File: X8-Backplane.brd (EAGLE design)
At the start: 101.9 x 101.6 mm, 17 parts

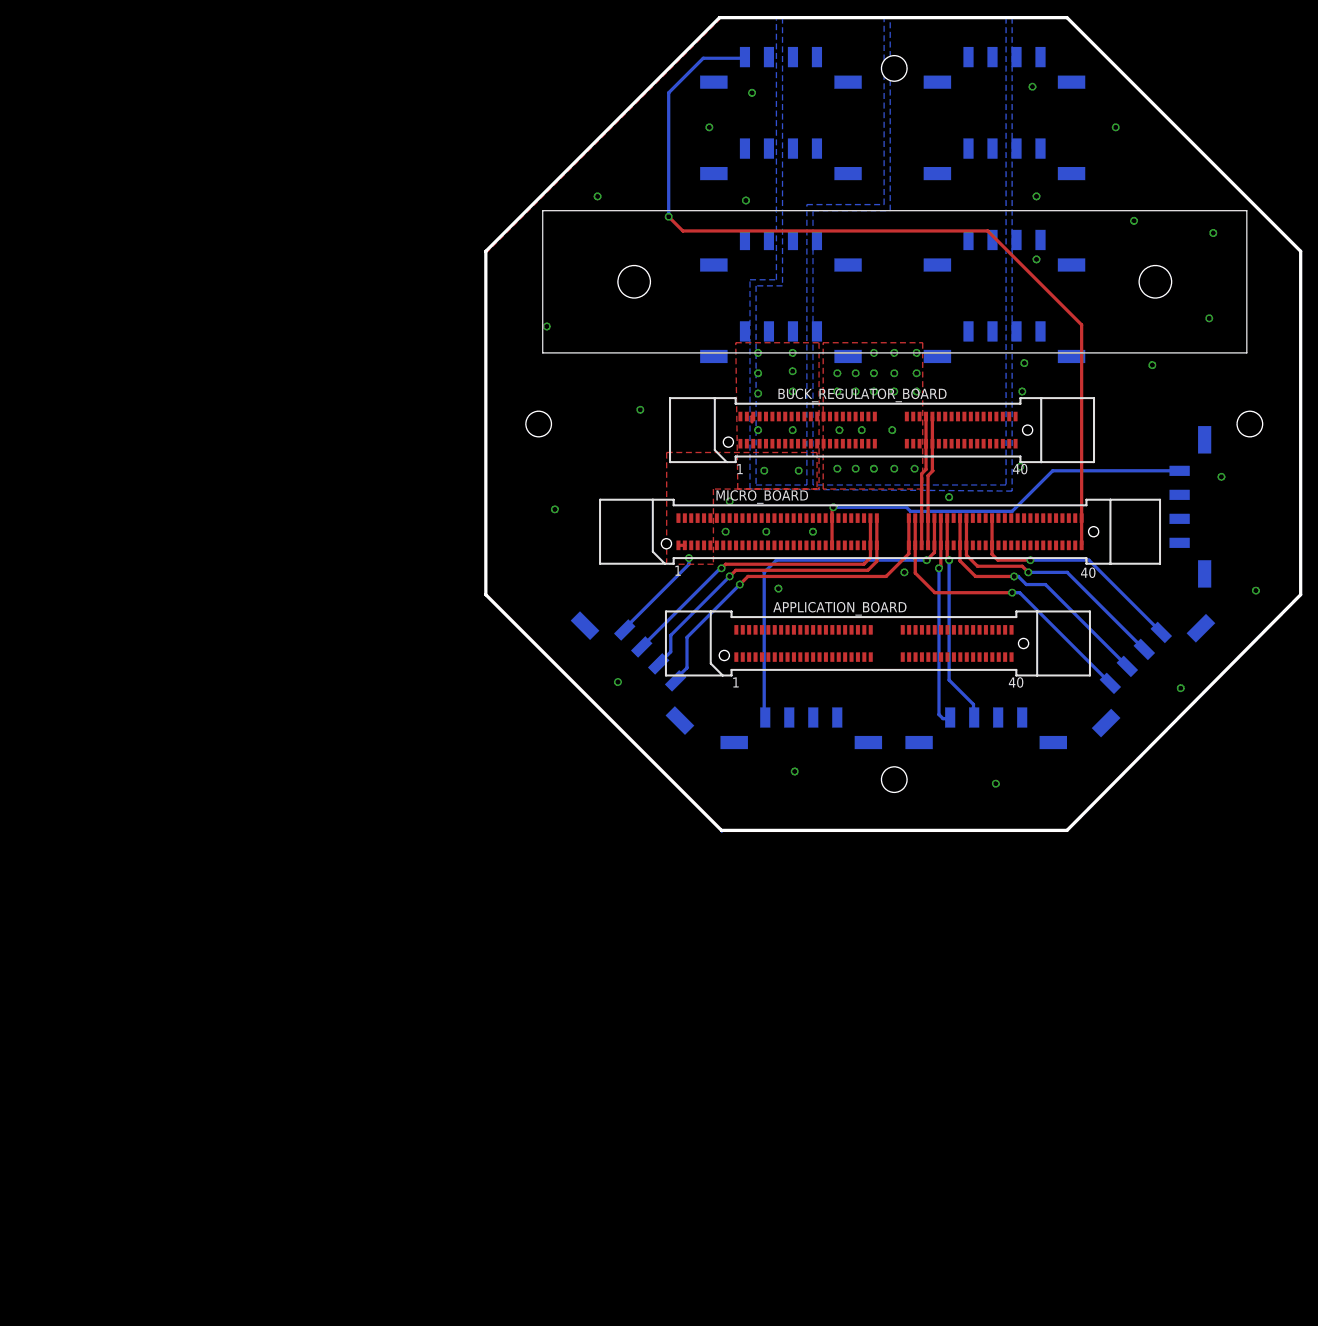
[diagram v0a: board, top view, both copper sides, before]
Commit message: Finished the backplane
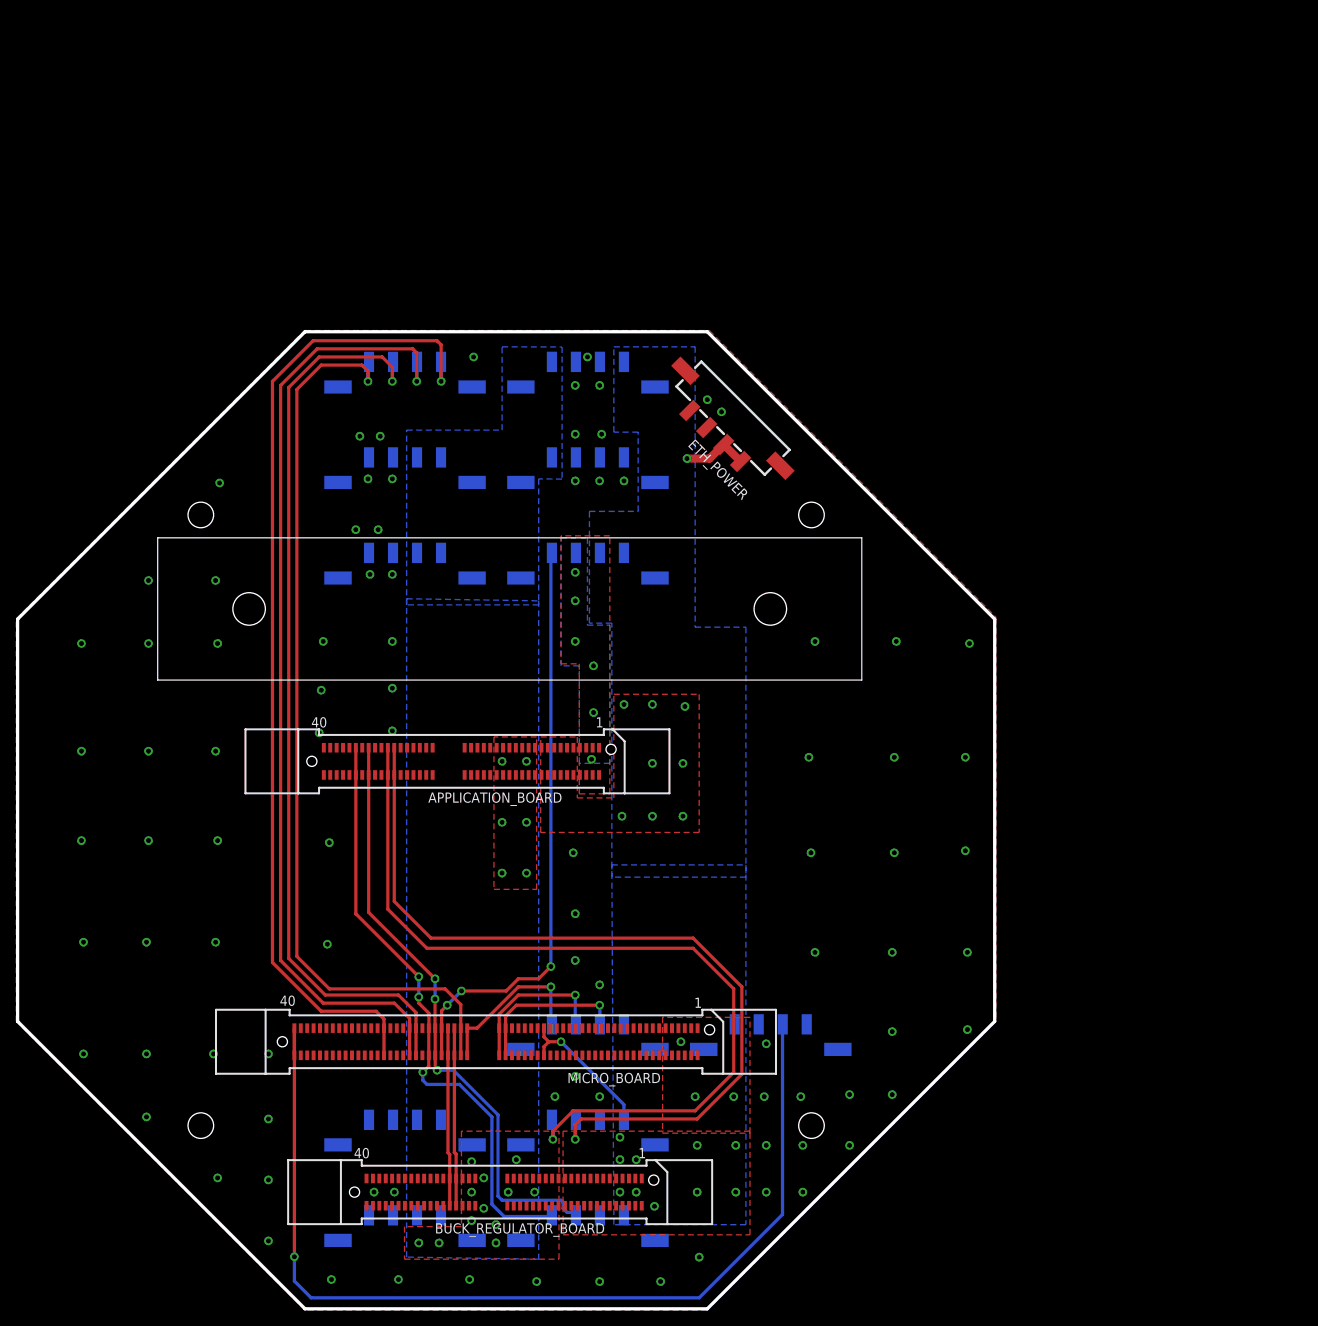
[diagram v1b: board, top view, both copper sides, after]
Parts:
- removed MA5N_CAM_POW: MICRO-FIT-4-SMD-PART, Connectors:MICRO-FIT-4-SMD
- added MAIN_CAM_POW: MICRO-FIT-4-SMD-PART, Connectors:MICRO-FIT-4-SMD
- moved POWER_INPUT 143.1 mm to (-2.54, -53.3)
- moved SOLENOID_POWER 123.8 mm to (-2.54, -41.4)
- moved EXTRA_SERVO 120.9 mm to (43.2, -29.5)
- moved TEMP_SENSOR 113.2 mm to (20.3, -41.4), turned to 0 degrees
- moved BUCK_REGULATOR_BOARD 106.1 mm to (-0.25, -46.5), turned to 180 degrees
- moved NAV_COM 95.6 mm to (-2.54, 53.3), turned to 0 degrees
- moved SEC_CAM_2 90.4 mm to (-2.54, 29.5)
- moved SEC_CAM_1 90.1 mm to (-2.54, 41.4)
- moved MICRO_BOARD 79.8 mm to (-1.27, -27.7), turned to 180 degrees
- moved BRICKS_COM 79.7 mm to (20.3, -53.3)
- moved APPLICATION_BOARD 53.6 mm to (-5.59, 7.37), turned to 180 degrees
- moved U$18 46.1 mm to (44.5, 35.3), turned to 180 degrees
- moved SOLENOID_DATA 40.2 mm to (20.3, -29.5), turned to 0 degrees
- moved ETH_POWER 37.3 mm to (36.1, 43.7), flipped to the top, turned to 135 degrees
- moved MAIN_CAM_DATA 33.7 mm to (20.3, 29.5)
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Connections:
- net +12V: now also APPLICATION_BOARD.21, APPLICATION_BOARD.22, APPLICATION_BOARD.23, APPLICATION_BOARD.24, APPLICATION_BOARD.25, APPLICATION_BOARD.26, APPLICATION_BOARD.27, APPLICATION_BOARD.28, APPLICATION_BOARD.29, APPLICATION_BOARD.30, APPLICATION_BOARD.31, APPLICATION_BOARD.32, APPLICATION_BOARD.33, APPLICATION_BOARD.34, MAIN_CAM_POW.C4, NAV_POWER.C4, POWER_INPUT.C1, POWER_INPUT.C2, SEC_CAM_1.C1, SEC_CAM_1.C2, SEC_CAM_2.C1, SEC_CAM_2.C2, SOLENOID_POWER.C1, SOLENOID_POWER.C2; no longer MA5N_CAM_POW.C1, NAV_POWER.C1, POWER_INPUT.C3, POWER_INPUT.C4, SEC_CAM_1.C3, SEC_CAM_1.C4, SEC_CAM_2.C3, SEC_CAM_2.C4, SOLENOID_POWER.C3, SOLENOID_POWER.C4
- net +3V3: now also APPLICATION_BOARD.57, APPLICATION_BOARD.58
- net +5V: now also APPLICATION_BOARD.10, APPLICATION_BOARD.11, APPLICATION_BOARD.12, APPLICATION_BOARD.13, APPLICATION_BOARD.14, APPLICATION_BOARD.15, APPLICATION_BOARD.16, APPLICATION_BOARD.17, APPLICATION_BOARD.18, APPLICATION_BOARD.19, APPLICATION_BOARD.20, APPLICATION_BOARD.9, EXTRA_SERVO.C4, MAIN_CAM_DATA.C1, MAIN_CAM_DATA.C2, NAV_POWER.C1, SOLENOID_DATA.C1; no longer EXTRA_SERVO.C2, MA5N_CAM_POW.C2, MA5N_CAM_POW.C3, NAV_POWER.C2, SOLENOID_DATA.C4
- net CANH: now also APPLICATION_BOARD.69, APPLICATION_BOARD.70, BRICKS_COM.C4; no longer BRICKS_COM.C3
- net CANL: now also APPLICATION_BOARD.65, APPLICATION_BOARD.66, BRICKS_COM.C3; no longer BRICKS_COM.C4
- net CLK: now also SOLENOID_DATA.C3; no longer SOLENOID_DATA.C2
- net DATA: now also SOLENOID_DATA.C4; no longer SOLENOID_DATA.C1
- net ENABLE: now also SOLENOID_DATA.C2; no longer SOLENOID_DATA.C3
- net GND: now also APPLICATION_BOARD.37, APPLICATION_BOARD.38, APPLICATION_BOARD.39, APPLICATION_BOARD.40, APPLICATION_BOARD.41, APPLICATION_BOARD.42, APPLICATION_BOARD.43, APPLICATION_BOARD.44, APPLICATION_BOARD.45, APPLICATION_BOARD.46, APPLICATION_BOARD.47, APPLICATION_BOARD.48, APPLICATION_BOARD.49, APPLICATION_BOARD.50, APPLICATION_BOARD.51, APPLICATION_BOARD.52, MAIN_CAM_POW.C1, MAIN_CAM_POW.C2, MAIN_CAM_POW.C3, NAV_POWER.C2, POWER_INPUT.C3, POWER_INPUT.C4, SEC_CAM_1.C3, SEC_CAM_1.C4, SEC_CAM_2.C3, SEC_CAM_2.C4, SOLENOID_POWER.C3, SOLENOID_POWER.C4; no longer MA5N_CAM_POW.C4, MAIN_CAM_DATA.C1, MAIN_CAM_DATA.C2, NAV_POWER.C4, POWER_INPUT.C1, POWER_INPUT.C2, SEC_CAM_1.C1, SEC_CAM_1.C2, SEC_CAM_2.C1, SEC_CAM_2.C2, SOLENOID_POWER.C1, SOLENOID_POWER.C2
- net LED_PWM: now also APPLICATION_BOARD.1, APPLICATION_BOARD.2, APPLICATION_BOARD.3, APPLICATION_BOARD.4, APPLICATION_BOARD.5, APPLICATION_BOARD.6, APPLICATION_BOARD.7, APPLICATION_BOARD.8
- net SECOND_SERVO: now also EXTRA_SERVO.C2; no longer EXTRA_SERVO.C4
- net TEMP_DATA: now also APPLICATION_BOARD.59, APPLICATION_BOARD.60
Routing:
- net TEMP_DATA: track 0.00 -> 107.1 mm, vias 0 -> 1
- net +3V3: track 0.00 -> 105.7 mm, vias 0 -> 1
- net SONAR_DAC: track 29.7 -> 124.4 mm
- net NAV_SCL: track 31.7 -> 120.8 mm
- net NAV_SDA: track 31.7 -> 114.7 mm
- net SONAR_PWM: track 37.0 -> 114.4 mm
- net CANH: track 26.3 -> 75.3 mm, vias 1 -> 3
- net CANL: track 26.3 -> 75.1 mm, vias 1 -> 3
- net BACK_UP_TEMP_DATA: track 50.4 -> 18.4 mm
- net MAIN_SERVO: track 44.8 -> 73.3 mm, vias 1 -> 3
- net DATA: track 42.5 -> 20.7 mm
- net CLK: track 39.2 -> 19.3 mm
- net ENABLE: track 38.1 -> 19.7 mm
- net SECOND_SERVO: track 111.6 -> 125.0 mm
- net BUCK_SDA: track 16.3 -> 22.3 mm
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- added copper zone on layer 1, net LED_PWM
- added copper zone on layer 16, net LED_PWM
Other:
- board size 101.9 x 101.6 mm -> 122.1 x 122.1 mm
